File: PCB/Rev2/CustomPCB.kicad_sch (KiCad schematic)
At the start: 28 parts, among them J1 Conn_01x06, J2 Conn_01x02, J3 Conn_01x03, Q1 AO3401A, SW1 RotaryEncoder, U1 PMW3610, U2 TLV74318PDBVR, U3 SuperMini nRF52840

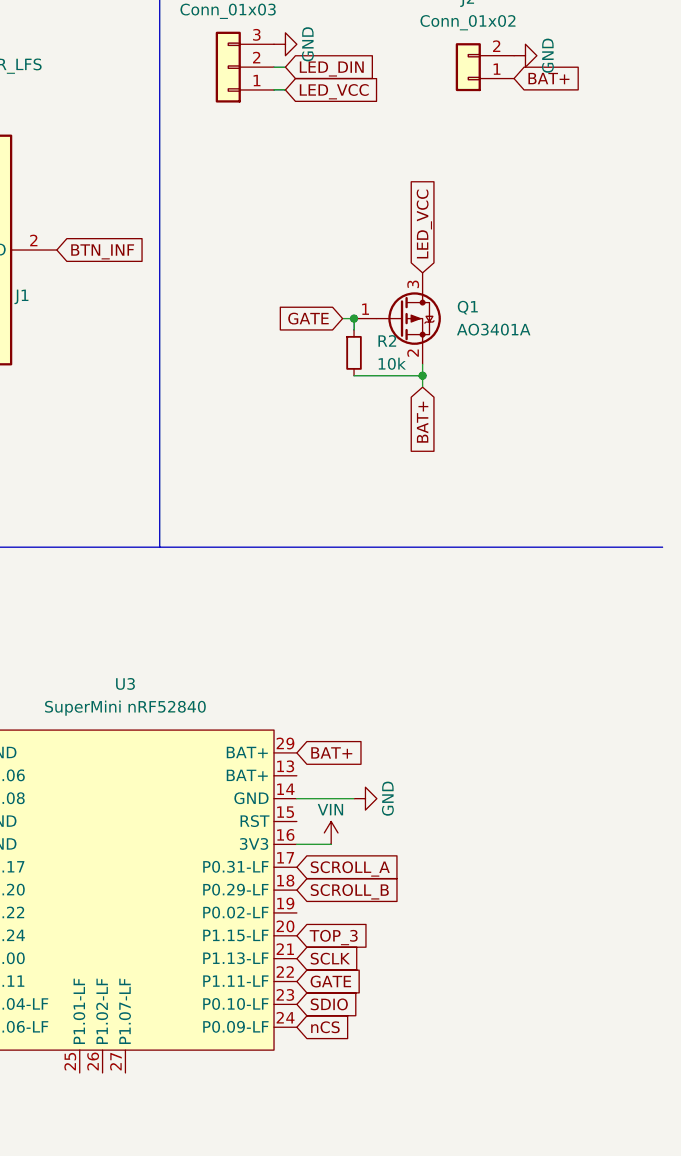
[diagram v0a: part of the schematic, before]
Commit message: Update Rev2 and documentation
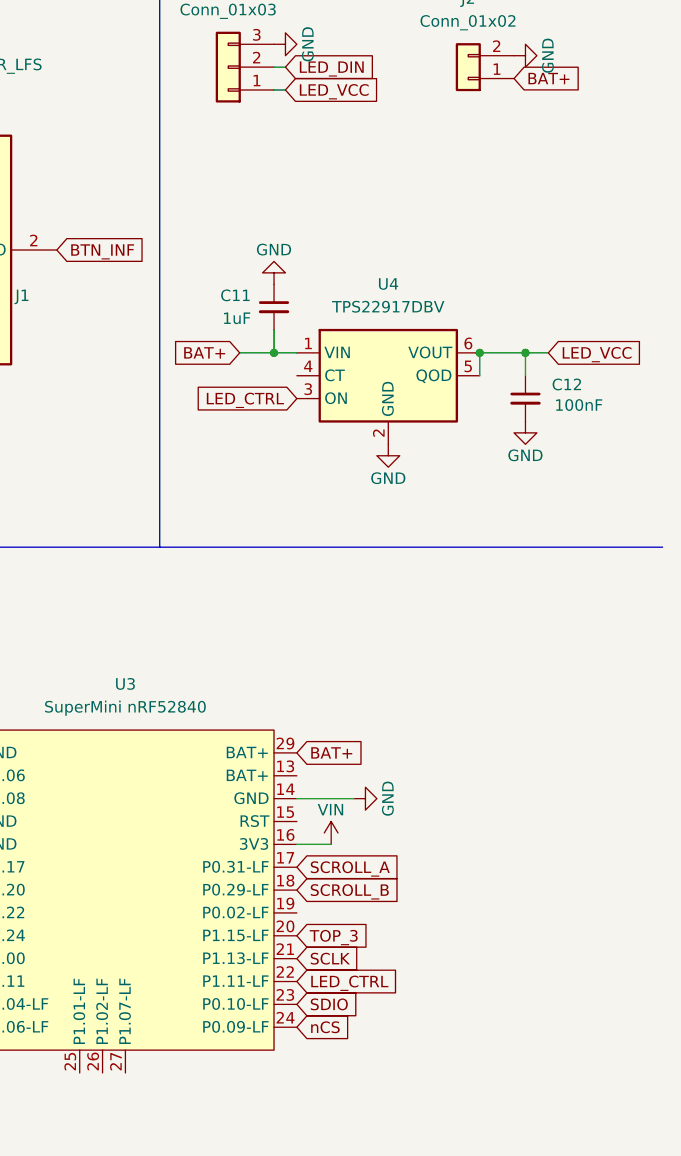
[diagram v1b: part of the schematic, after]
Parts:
- removed Q1: AO3401A, Package_TO_SOT_SMD:SOT-23, symbol Transistor_FET:AO3401A
- removed R2: 10k, Resistor_SMD:R_0603_1608Metric, symbol Device:R_Small
- added C11: 1uF, Capacitor_SMD:C_0603_1608Metric, symbol Device:C_Small
- added C12: 100nF, Capacitor_SMD:C_0603_1608Metric, symbol Device:C_Small
- added U4: TPS22917DBV, Package_TO_SOT_SMD:SOT-23-6, symbol Power_Management:TPS22917DBV
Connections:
- net BAT+: now also C11.2, U4.1 (VIN)
- net GND: now also C11.1, C12.2, U4.2 (GND)
- net LED_VCC: now also C12.1, U4.5 (QOD), U4.6 (VOUT)
- net GATE renamed LED_CTRL
- net LED_CTRL: now also U4.3 (ON)
